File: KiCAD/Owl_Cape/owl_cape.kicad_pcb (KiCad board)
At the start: 2 copper layers, 232 x 146 mm, 114 parts, among them IC1 SN74AHC245N, IC2 SN74HC244N, IC3 Raspberry_Pi_Zero_2_W__v1.0_, J1 G D V, J10 G D V, J11 G D V, J12 G D V, J13 G D V, J14 G D V, J15 G D V, J16 G D V, J17 OLED, J18 8P8C_LED_Shielded, J19 8P8C_LED_Shielded, J2 G D V, J20 8P8C_LED_Shielded, J22 9-16 In, J23 1-8 In, J3 G D V, J30 Conn_02x20_Odd_Even_MountingP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, J4 G D V, J5 G D V, J6 G D V, J7 G D V, J8 G D V, J9 G D V, Q1 MMDT5401, Q2 DMG2302U, SW1 Enter BTN, SW2 Down BTN, U1 AT24C256C, U2 D-SUN_MP1584_BUCK, U3 TZT_Original_0.96_inch_oled_I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, U4 LAN7500-ABJZ

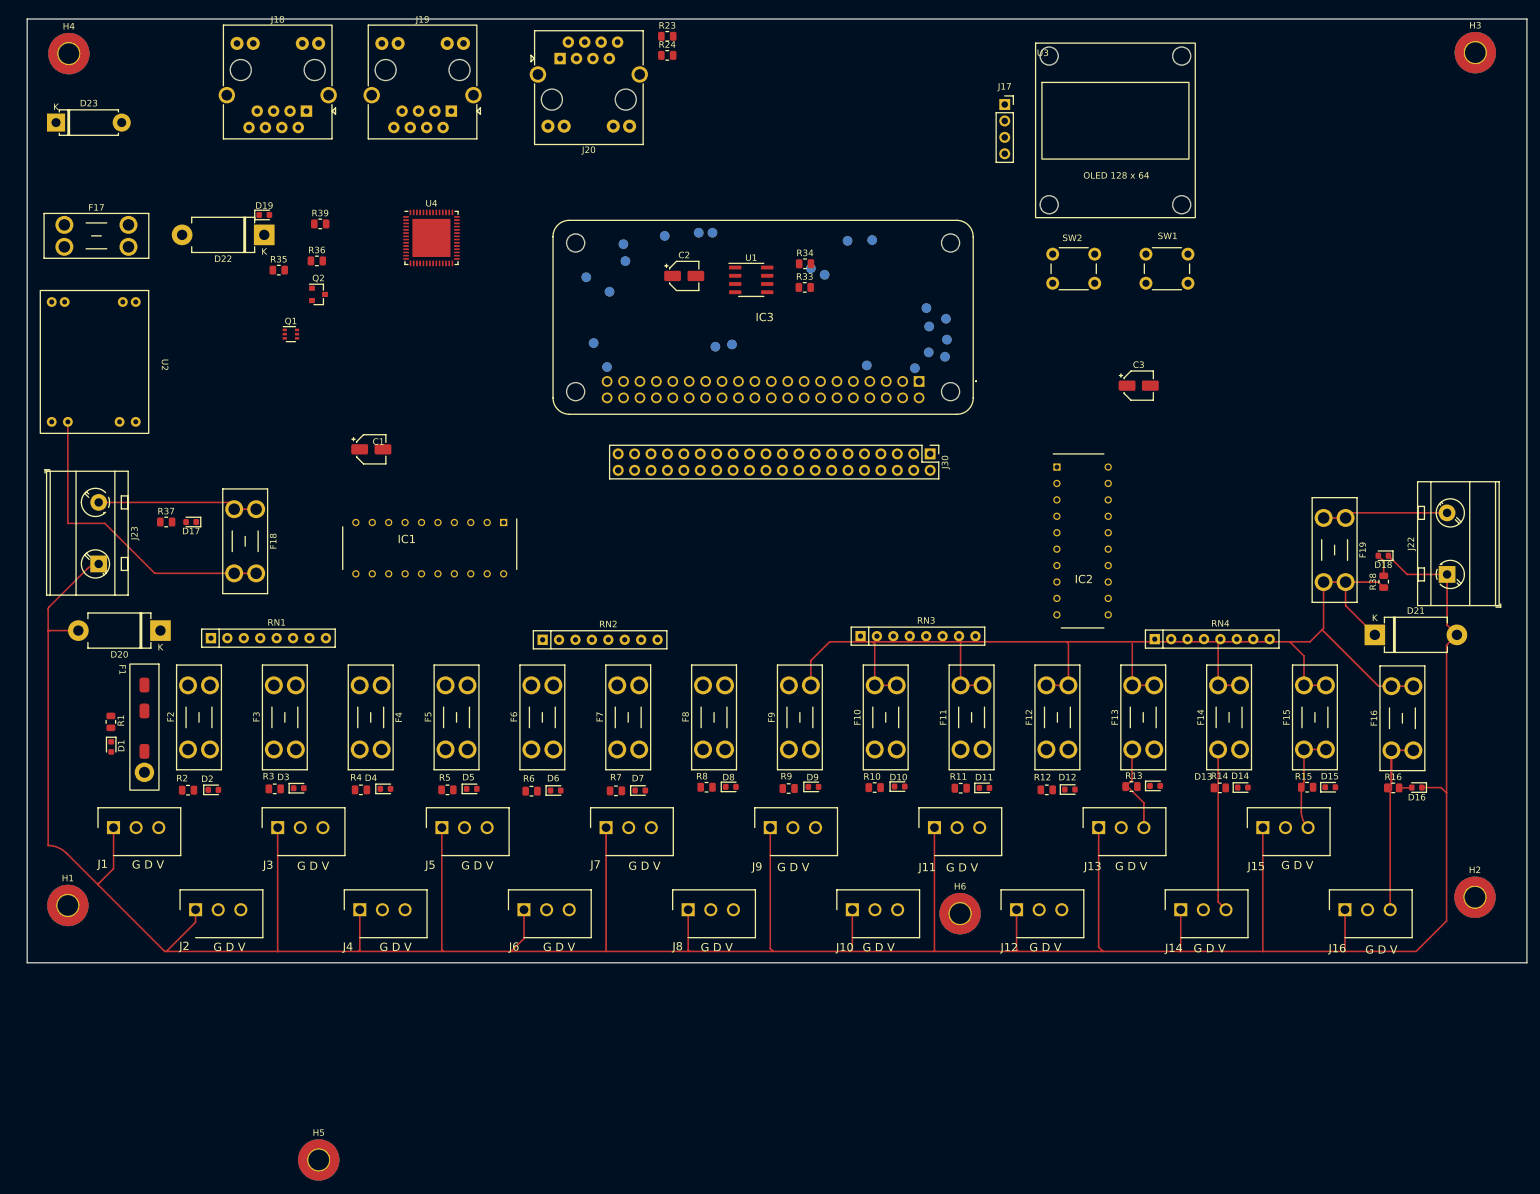
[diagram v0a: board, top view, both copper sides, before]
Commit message: major update to layout
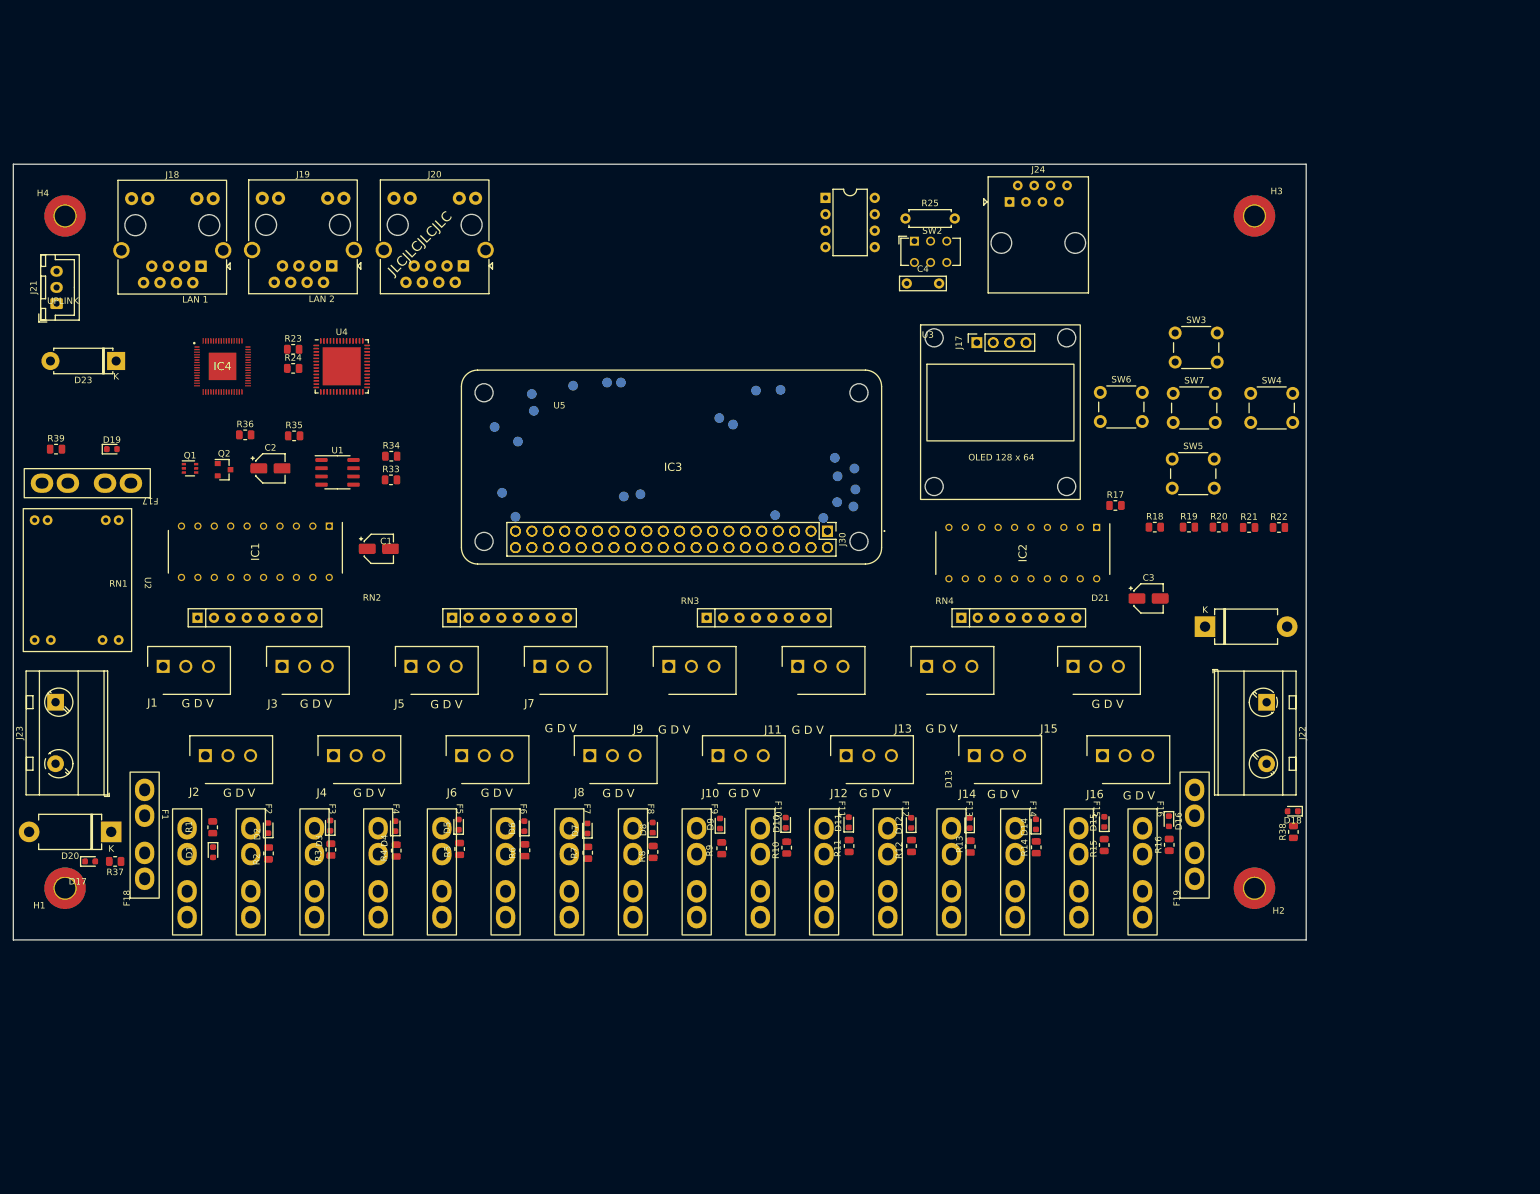
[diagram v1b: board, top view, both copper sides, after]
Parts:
- removed D22: SB5100, Diode_THT:D_DO-201AD_P12.70mm_Horizontal
- removed H5, H6: M3 MountingHole, MountingHole:MountingHole_3.2mm_M3_Pad_TopBottom
- removed SW1: Enter BTN, Button_Switch_THT:SW_PUSH_6mm
- added C4: 0.1uF, Capacitor_THT:C_Rect_L7.0mm_W2.0mm_P5.00mm, F.Cu at (183.1, 54.9)
- added IC4: KSZ8794CNXIC, SamacSys_Parts:QFN40P800X800X90-65N, F.Cu at (77.2, 67.7)
- added J21: GPIO TRG, Connector_JST:JST_XH_B3B-XH-A_1x03_P2.50mm_Vertical, F.Cu at (51.5, 58.0)
- added J24: DMX1 RJ45, Connector_RJ:RJ45_Amphenol_54602-x08_Horizontal, F.Cu at (199.0, 42.3)
- added R17: Pull_Up_resistor, Resistor_SMD:R_0805_2012Metric, F.Cu at (215.3, 89.3)
- added R18: 2.2K, Resistor_SMD:R_0805_2012Metric, F.Cu at (221.4, 92.6)
- added R19: 2.2K, Resistor_SMD:R_0805_2012Metric, F.Cu at (226.7, 92.6)
- added R20: 2.2K, Resistor_SMD:R_0805_2012Metric, F.Cu at (231.3, 92.6)
- added R21: 2.2K, Resistor_SMD:R_0805_2012Metric, F.Cu at (236.0, 92.7)
- added R22: 2.2K, Resistor_SMD:R_0805_2012Metric, F.Cu at (240.6, 92.7)
- added R25: 120, Resistor_THT:R_Axial_DIN0207_L6.3mm_D2.5mm_P7.62mm_Horizontal, F.Cu at (182.9, 44.9)
- added SW3: SW_UP, Button_Switch_THT:SW_PUSH_6mm, F.Cu at (224.6, 62.6)
- added SW4: SW_RIGHT, Button_Switch_THT:SW_PUSH_6mm, F.Cu at (236.3, 71.9)
- added SW5: SW_DOWN, Button_Switch_THT:SW_PUSH_6mm, F.Cu at (224.1, 82.1)
- added SW6: SW_LEFT, Button_Switch_THT:SW_PUSH_6mm, F.Cu at (213.0, 71.8)
- added SW7: SW_ENTER, Button_Switch_THT:SW_PUSH_6mm, F.Cu at (224.3, 71.9)
- added U5: UA9638CP, Package_DIP:DIP-8_W7.62mm, F.Cu at (170.5, 41.7)
- F10: value P2 -> P1; footprint Fuse:Fuseholder_Blade_Mini_Keystone_3568 -> Stuart_BESPOKE:Medium Auto Fuse Holder
- F11: value P3 -> P1; footprint Fuse:Fuseholder_Blade_Mini_Keystone_3568 -> Stuart_BESPOKE:Medium Auto Fuse Holder
- F12: value P4 -> P1; footprint Fuse:Fuseholder_Blade_Mini_Keystone_3568 -> Stuart_BESPOKE:Medium Auto Fuse Holder
- F13: value P5 -> P1; footprint Fuse:Fuseholder_Blade_Mini_Keystone_3568 -> Stuart_BESPOKE:Medium Auto Fuse Holder
- F14: value P6 -> P1; footprint Fuse:Fuseholder_Blade_Mini_Keystone_3568 -> Stuart_BESPOKE:Medium Auto Fuse Holder
- F15: value P7 -> P1; footprint Fuse:Fuseholder_Blade_Mini_Keystone_3568 -> Stuart_BESPOKE:Medium Auto Fuse Holder
- F16: value P8 -> P1; footprint Fuse:Fuseholder_Blade_Mini_Keystone_3568 -> Stuart_BESPOKE:Medium Auto Fuse Holder
- F17, F18, F19, F2, F3, F4, F5, F6, F7, F8, F9: footprint Fuse:Fuseholder_Blade_Mini_Keystone_3568 -> Stuart_BESPOKE:Medium Auto Fuse Holder
- IC2: value SN74HC244N -> SN74AHC245N
- J18: value 8P8C_LED_Shielded -> UPLINK
- J19: value 8P8C_LED_Shielded -> LAN 1
- J20: value 8P8C_LED_Shielded -> LAN 2
- SW2: value Down BTN -> DMX_LOR_Select; footprint Button_Switch_THT:SW_PUSH_6mm -> Button_Switch_THT:SW_CuK_JS202011CQN_DPDT_Straight
- moved R23 75.5 mm to (88.1, 65.1)
- moved R24 75.5 mm to (88.1, 68.0)
- moved C2 70.6 mm to (84.6, 83.5)
- moved R33 70.6 mm to (103.3, 85.3)
- moved R34 70.6 mm to (103.3, 81.6)
- moved U1 70.6 mm to (95.0, 84.1)
- moved F19 64.1 mm to (225.3, 150.0), turned to 90 degrees
- moved F18 63.2 mm to (62.9, 150.0), turned to 90 degrees
- moved D17 54.8 mm to (56.7, 144.3), turned to 0 degrees
- moved R39 53.7 mm to (51.5, 80.5)
- moved R37 53.1 mm to (60.6, 144.3), turned to 180 degrees
- moved U3 47.1 mm to (185.2, 61.3)
- moved J16 44.4 mm to (213.3, 127.9)
- moved F17 44.3 mm to (66.0, 88.1), turned to 180 degrees
- moved D19 43.2 mm to (60.1, 80.5)
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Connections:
- F1 pad 1: Net-(F1-Pad1) -> VIN1
- F1 pad 3: (no net) -> Net-(F1-Pad3)
- F1 pad 4: (no net) -> Net-(F1-Pad3)
- F10 pad 1: Net-(F10-Pad1) -> VIN2
- F11 pad 1: Net-(F11-Pad1) -> VIN2
- F12 pad 1: Net-(F12-Pad1) -> VIN2
- F13 pad 1: Net-(F13-Pad1) -> VIN2
- F14 pad 1: Net-(F14-Pad1) -> VIN2
- F15 pad 1: Net-(F15-Pad1) -> VIN2
- F16 pad 1: Net-(F16-Pad1) -> VIN2
- F17 pad 2: +5V -> V5
- F18 pad 2: VIN1 -> V1
- F19 pad 2: VIN2 -> V2
- F2 pad 1: Net-(F2-Pad1) -> VIN1
- F3 pad 1: Net-(F3-Pad1) -> VIN1
- F4 pad 1: Net-(F4-Pad1) -> VIN1
- F5 pad 1: Net-(F5-Pad1) -> VIN1
- F6 pad 1: Net-(F6-Pad1) -> VIN1
- F7 pad 1: Net-(F7-Pad1) -> VIN1
- F8 pad 1: Net-(F8-Pad1) -> VIN1
- F9 pad 1: Net-(F9-Pad1) -> VIN2
- IC1 pad 1: GND -> +5V
- IC2 pad 1: GND -> +5V
- IC2 pad 11: DATA13 -> Net-(IC2-Pad11)
- IC2 pad 13: DATA14 -> Net-(IC2-Pad13)
- IC2 pad 15: DATA15 -> Net-(IC2-Pad15)
- IC2 pad 17: DATA16 -> Net-(IC2-Pad17)
- IC2 pad 2: DATA9 -> DATA16
- IC2 pad 3: Net-(IC2-Pad3) -> DATA15
- IC2 pad 4: DATA10 -> DATA14
- IC2 pad 5: Net-(IC2-Pad5) -> DATA13
- IC2 pad 6: DATA11 -> DATA12
- IC2 pad 7: Net-(IC2-Pad7) -> DATA11
- IC2 pad 8: DATA12 -> DATA10
- IC2 pad 9: Net-(IC2-Pad9) -> DATA9
- J1 pad 3: Net-(F1-Pad1) -> Net-(F1-Pad3)
- J10 pad 3: Net-(F10-Pad1) -> Net-(F10-Pad3)
- J11 pad 3: Net-(F11-Pad1) -> Net-(F11-Pad3)
- J12 pad 3: Net-(F12-Pad1) -> Net-(F12-Pad3)
- J13 pad 3: Net-(F13-Pad1) -> Net-(F13-Pad3)
- J14 pad 3: Net-(F14-Pad1) -> Net-(F14-Pad3)
- J15 pad 3: Net-(F15-Pad1) -> Net-(F15-Pad3)
- J16 pad 3: Net-(F16-Pad1) -> Net-(F16-Pad3)
- J18 pad 1: Net-(J18-Pad1) -> unconnected-(J18-Pad1)
- J18 pad 10: Net-(J18-Pad10) -> unconnected-(J18-Pad10)
- J18 pad 11: GND -> unconnected-(J18-Pad11)
- J18 pad 12: Net-(J18-Pad12) -> unconnected-(J18-Pad12)
- J18 pad 2: Net-(J18-Pad2) -> unconnected-(J18-Pad2)
- J18 pad 3: Net-(J18-Pad3) -> unconnected-(J18-Pad3)
- J18 pad 4: Net-(J18-Pad4) -> unconnected-(J18-Pad4)
- J18 pad 5: Net-(J18-Pad5) -> unconnected-(J18-Pad5)
- J18 pad 6: Net-(J18-Pad6) -> unconnected-(J18-Pad6)
- J18 pad 7: Net-(J18-Pad7) -> unconnected-(J18-Pad7)
- J18 pad 8: Net-(J18-Pad8) -> unconnected-(J18-Pad8)
- J18 pad 9: GND -> unconnected-(J18-Pad9)
- J18 pad SH: GND -> unconnected-(J18-PadSH)
- J2 pad 3: Net-(F2-Pad1) -> Net-(F2-Pad3)
- J3 pad 3: Net-(F3-Pad1) -> Net-(F3-Pad3)
- J30 pad 18: BTN1 -> DATA7
- J30 pad 22: BTN2 -> BTN1
- J30 pad 29: unconnected-(J30-Pad29) -> BTN_ARRAY_ANALOGUE_IN
- J30 pad 8: DATA7 -> TXD1
- J4 pad 3: Net-(F4-Pad1) -> Net-(F4-Pad3)
- J5 pad 3: Net-(F5-Pad1) -> Net-(F5-Pad3)
- J6 pad 3: Net-(F6-Pad1) -> Net-(F6-Pad3)
- J7 pad 3: Net-(F7-Pad1) -> Net-(F7-Pad3)
- J8 pad 3: Net-(F8-Pad1) -> Net-(F8-Pad3)
- J9 pad 3: Net-(F9-Pad1) -> Net-(F9-Pad3)
- R1 pad 1: Net-(F1-Pad1) -> Net-(F1-Pad3)
- R10 pad 1: Net-(F10-Pad1) -> Net-(F10-Pad3)
- R11 pad 1: Net-(F11-Pad1) -> Net-(F11-Pad3)
- R12 pad 1: Net-(F12-Pad1) -> Net-(F12-Pad3)
- R13 pad 1: Net-(F13-Pad1) -> Net-(F13-Pad3)
- R14 pad 1: Net-(F14-Pad1) -> Net-(F14-Pad3)
- R15 pad 1: Net-(F15-Pad1) -> Net-(F15-Pad3)
- R16 pad 1: Net-(F16-Pad1) -> Net-(F16-Pad3)
- R2 pad 1: Net-(F2-Pad1) -> Net-(F2-Pad3)
- R3 pad 1: Net-(F3-Pad1) -> Net-(F3-Pad3)
- R4 pad 1: Net-(F4-Pad1) -> Net-(F4-Pad3)
- R5 pad 1: Net-(F5-Pad1) -> Net-(F5-Pad3)
- R6 pad 1: Net-(F6-Pad1) -> Net-(F6-Pad3)
- R7 pad 1: Net-(F7-Pad1) -> Net-(F7-Pad3)
- R8 pad 1: Net-(F8-Pad1) -> Net-(F8-Pad3)
- R9 pad 1: Net-(F9-Pad1) -> Net-(F9-Pad3)
- RN3 pad 1: Net-(IC2-Pad18) -> Net-(IC2-Pad11)
- RN3 pad 3: Net-(IC2-Pad16) -> Net-(IC2-Pad12)
- RN3 pad 5: Net-(IC2-Pad14) -> Net-(IC2-Pad13)
- RN3 pad 7: Net-(IC2-Pad12) -> Net-(IC2-Pad14)
- RN4 pad 1: Net-(IC2-Pad9) -> Net-(IC2-Pad15)
- RN4 pad 3: Net-(IC2-Pad7) -> Net-(IC2-Pad16)
- RN4 pad 5: Net-(IC2-Pad5) -> Net-(IC2-Pad17)
- RN4 pad 7: Net-(IC2-Pad3) -> Net-(IC2-Pad18)
- SW2 pad 1: GND -> Net-(J24-Pad4)
- SW2 pad 2: BTN2 -> /Serial_Diffs/DMX1+
- U4 pad 31: Net-(J18-Pad10) -> unconnected-(U4-Pad31)
- U4 pad 32: Net-(J18-Pad12) -> unconnected-(U4-Pad32)
- U4 pad 43: Net-(J18-Pad1) -> unconnected-(U4-Pad43)
- U4 pad 44: Net-(J18-Pad2) -> unconnected-(U4-Pad44)
- U4 pad 46: Net-(J18-Pad3) -> unconnected-(U4-Pad46)
- U4 pad 47: Net-(J18-Pad4) -> unconnected-(U4-Pad47)
- U4 pad 51: Net-(J18-Pad5) -> unconnected-(U4-Pad51)
- U4 pad 52: Net-(J18-Pad6) -> unconnected-(U4-Pad52)
- U4 pad 54: Net-(J18-Pad7) -> unconnected-(U4-Pad54)
- U4 pad 55: Net-(J18-Pad8) -> unconnected-(U4-Pad55)
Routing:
- net GND: track 545.7 -> 0.00 mm
- net VIN2: track 191.5 -> 0.00 mm
- net VIN1: track 48.0 -> 0.00 mm
- net Net-(F16-Pad1): track 34.2 -> 0.00 mm
- net V1: track 25.4 -> 0.00 mm
- net Net-(F14-Pad1): track 25.3 -> 0.00 mm
- net V2: track 19.4 -> 0.00 mm
- net Net-(F15-Pad1): track 15.9 -> 0.00 mm
- net Net-(F13-Pad1): track 13.9 -> 0.00 mm
- net Net-(D18-Pad2): track 3.45 -> 0.00 mm
- net Net-(D16-Pad2): track 1.98 -> 0.00 mm
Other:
- board size 232 x 146 mm -> 200 x 120 mm
- board text added: "JLCJLCJLCJLC"
